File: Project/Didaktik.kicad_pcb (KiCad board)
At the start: 2 copper layers, 209.6 x 76.2 mm, 129 parts, among them J1 Conn_01x04_MountingPin, J2 AVR-ISP-6, J3 Conn_01x03, Q1 2N2222, SW1 SW_Push_45deg, SW10 SW_Push_45deg, SW11 SW_Push_45deg, SW12 SW_Push_45deg, SW13 SW_Push_45deg, SW14 SW_Push_45deg, SW15 SW_Push_45deg, SW16 SW_Push_45deg, SW17 SW_Push_45deg, SW18 SW_Push_45deg, SW19 SW_Push_45deg, SW2 SW_Push_45deg, SW20 SW_Push_45deg, SW21 SW_Push_45deg, SW22 SW_Push_45deg, SW23 SW_Push_45deg, SW24 SW_Push_45deg, SW25 SW_Push_45deg, SW26 SW_Push_45deg, SW27 SW_Push_45deg, SW28 SW_Push_45deg, SW29 SW_Push_45deg, SW3 SW_Push_45deg, SW30 SW_Push_45deg, SW31 SW_Push_45deg, SW31a1 SW_Push_45deg, SW32 SW_Push_45deg, SW32a1 SW_Push_45deg, SW33 SW_Push_45deg, SW33a1 SW_Push_45deg, SW34 SW_Push_45deg, SW34a1 SW_Push_45deg, SW34b1 SW_Push_45deg, SW35 SW_Push_45deg, SW35a1 SW_Push_45deg, SW35b1 SW_Push_45deg, SW35c1 SW_Push_45deg, SW36 SW_Push_45deg, SW36a1 SW_Push_45deg, SW36b1 SW_Push_45deg, SW36c1 SW_Push_45deg, SW37 SW_Push_45deg, SW37a1 SW_Push_45deg, SW37b1 SW_Push_45deg, SW38 SW_Push_45deg, SW38a1 SW_Push_45deg, SW39 SW_Push_45deg, SW39a1 SW_Push_45deg, SW4 SW_Push_45deg, SW40 SW_Push_45deg, SW40a1 SW_Push_45deg, SW41 RotaryEncoder_Switch, SW42 RotaryEncoder_Switch, SW5 SW_Push_45deg, SW6 SW_Push_45deg, SW7 SW_Push_45deg, SW8 SW_Push_45deg, SW9 SW_Push_45deg, U1 ATmega32U4-M, Y1 Crystal_GND24_Small

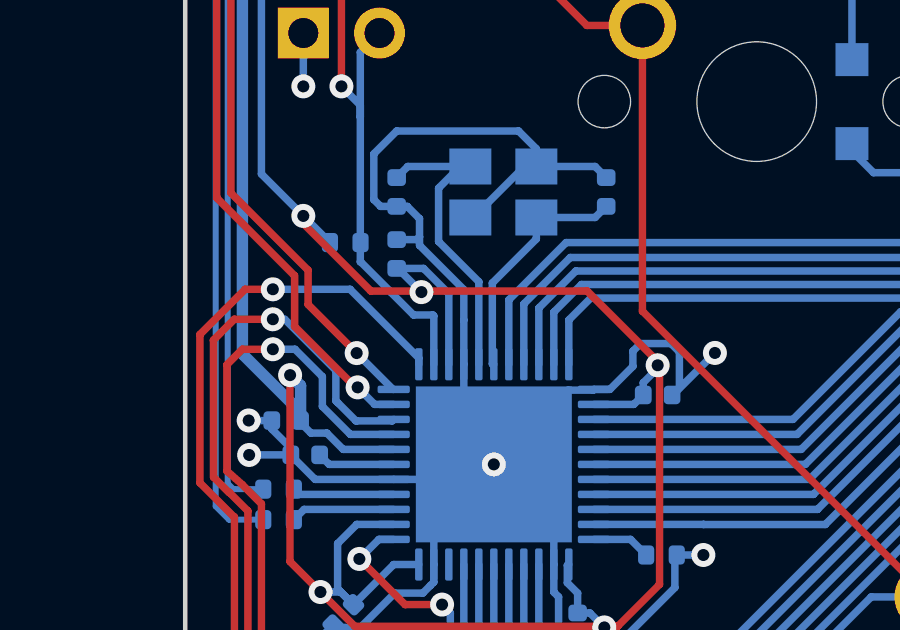
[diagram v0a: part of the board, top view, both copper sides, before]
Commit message: update
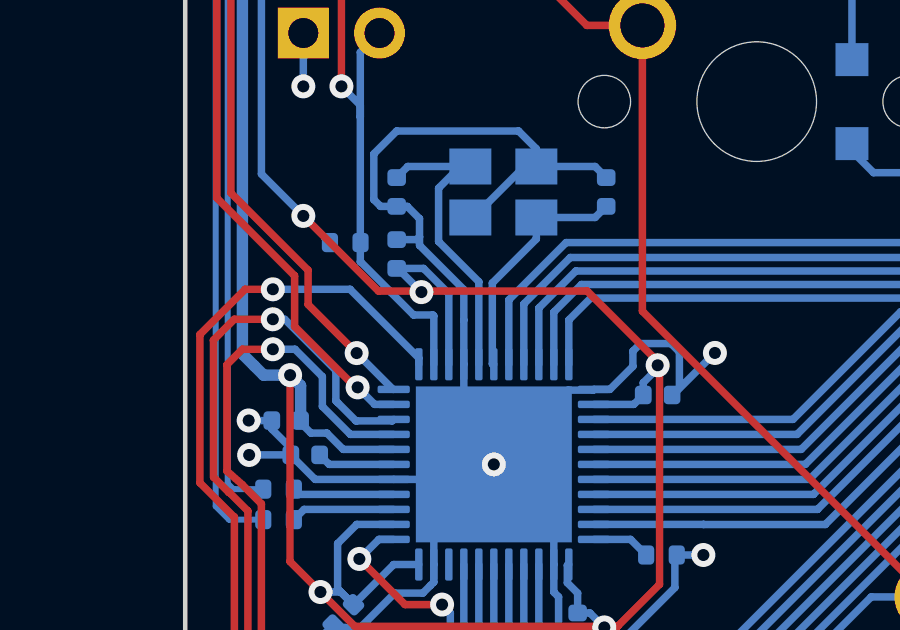
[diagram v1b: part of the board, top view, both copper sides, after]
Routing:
- net +5V: track 301.0 -> 300.0 mm
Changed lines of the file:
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@@
   (segment (start 233.172 39.116) (end 233.172 41.783) (width 0.2) (layer "B.Cu") (net 56))
   (segment (start 35.2425 69.445977) (end 35.246463 69.442014) (width 0.25) (layer "F.Cu") (net 57))
-  (segment (start 47.5615 69.05225) (end 45.1485 66.63925) (width 0.25) (layer "F.Cu") (net 57))
   (segment (start 46.1645 77.81525) (end 47.5615 76.41825) (width 0.25) (layer "F.Cu") (net 57))
-  (segment (start 37.93725 66.63925) (end 35.687 64.389) (width 0.25) (layer "F.Cu") (net 57))
   (segment (start 47.4985 69.114) (end 47.49975 69.114) (width 0.25) (layer "F.Cu") (net 57))
   (segment (start 47.49975 69.114) (end 47.5615 69.05225) (width 0.25) (layer "F.Cu") (net 57))
-  (segment (start 35.687 64.389) (end 35.687 64.135) (width 0.25) (layer "F.Cu") (net 57))
+  (segment (start 38.19125 66.63925) (end 45.1485 66.63925) (width 0.25) (layer "F.Cu") (net 57))
   (segment (start 35.2425 75.65625) (end 35.2425 69.445977) (width 0.25) (layer "F.Cu") (net 57))
+  (segment (start 45.1485 66.63925) (end 47.5615 69.05225) (width 0.25) (layer "F.Cu") (net 57))
   (segment (start 45.4025 77.81525) (end 46.1645 77.81525) (width 0.25) (layer "F.Cu") (net 57))
   (segment (start 37.4015 77.81525) (end 46.1645 77.81525) (width 0.25) (layer "F.Cu") (net 57))
   (segment (start 47.5615 76.41825) (end 47.5615 69.05225) (width 0.25) (layer "F.Cu") (net 57))
-  (segment (start 45.1485 66.63925) (end 37.93725 66.63925) (width 0.25) (layer "F.Cu") (net 57))
+  (segment (start 35.687 64.135) (end 38.19125 66.63925) (width 0.25) (layer "F.Cu") (net 57))
   (segment (start 35.2425 75.65625) (end 37.4015 77.81525) (width 0.25) (layer "F.Cu") (net 57))
   (via (at 35.246463 69.442014) (size 0.8) (drill 0.4) (layers "F.Cu" "B.Cu") (net 57))
@@
   (via (at 47.4985 69.114) (size 0.8) (drill 0.4) (layers "F.Cu" "B.Cu") (net 57))
   (via (at 39.624 66.675) (size 0.8) (drill 0.4) (layers "F.Cu" "B.Cu") (net 57))
+  (segment (start 34.053875 69.133625) (end 34.362264 69.442014) (width 0.381) (layer "B.Cu") (net 57))
   (segment (start 44.537 75.75525) (end 44.51375 75.75525) (width 0.25) (layer "B.Cu") (net 57))
   (segment (start 36.574 65.022) (end 35.687 64.135) (width 0.25) (layer "B.Cu") (net 57))
@@
   (segment (start 44.831 76.708) (end 44.831 77.371) (width 0.25) (layer "B.Cu") (net 57))
   (segment (start 47.4985 69.2145) (end 47.4985 69.114) (width 0.25) (layer "B.Cu") (net 57))
+  (segment (start 34.362264 69.442014) (end 35.246463 69.442014) (width 0.381) (layer "B.Cu") (net 57))
   (segment (start 35.941 71.374) (end 36.471859 71.374) (width 0.25) (layer "B.Cu") (net 57))
   (segment (start 38.7985 65.885) (end 38.834 65.885) (width 0.25) (layer "B.Cu") (net 57))
@@
   (segment (start 44.487 76.364) (end 44.831 76.708) (width 0.25) (layer "B.Cu") (net 57))
   (segment (start 34.29 62.738) (end 34.29 54.356) (width 0.25) (layer "B.Cu") (net 57))
-  (segment (start 35.5955 70.67525) (end 33.6565 68.73625) (width 0.381) (layer "B.Cu") (net 57))
   (segment (start 45.24 77.371) (end 45.72 77.851) (width 0.25) (layer "B.Cu") (net 57))
   (segment (start 44.487 75.782) (end 44.487 76.364) (width 0.25) (layer "B.Cu") (net 57))
@@
   (segment (start 36.471859 71.374) (end 37.015609 71.91775) (width 0.25) (layer "B.Cu") (net 57))
   (segment (start 34.29 54.356) (end 35.687 52.959) (width 0.25) (layer "B.Cu") (net 57))
+  (segment (start 34.053875 69.133625) (end 33.6565 68.73625) (width 0.381) (layer "B.Cu") (net 57))
   (segment (start 36.83 75.057) (end 36.83 76.564928) (width 0.25) (layer "B.Cu") (net 57))
   (segment (start 233.1735 50.8015) (end 233.807 50.168) (width 0.381) (layer "B.Cu") (net 57))
